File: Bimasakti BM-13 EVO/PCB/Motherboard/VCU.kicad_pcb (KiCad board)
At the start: 2 copper layers, 190.7 x 210 mm, 27 parts, among them J1 6437288-3, J10 power, J11 6437288-3, J2 12V, J3 3V3_1, J4 5V_5, J5 5V_1, J6 5V_2, J7 5V_3, J8 SIGNAL 1, J9 SIGNAL 2

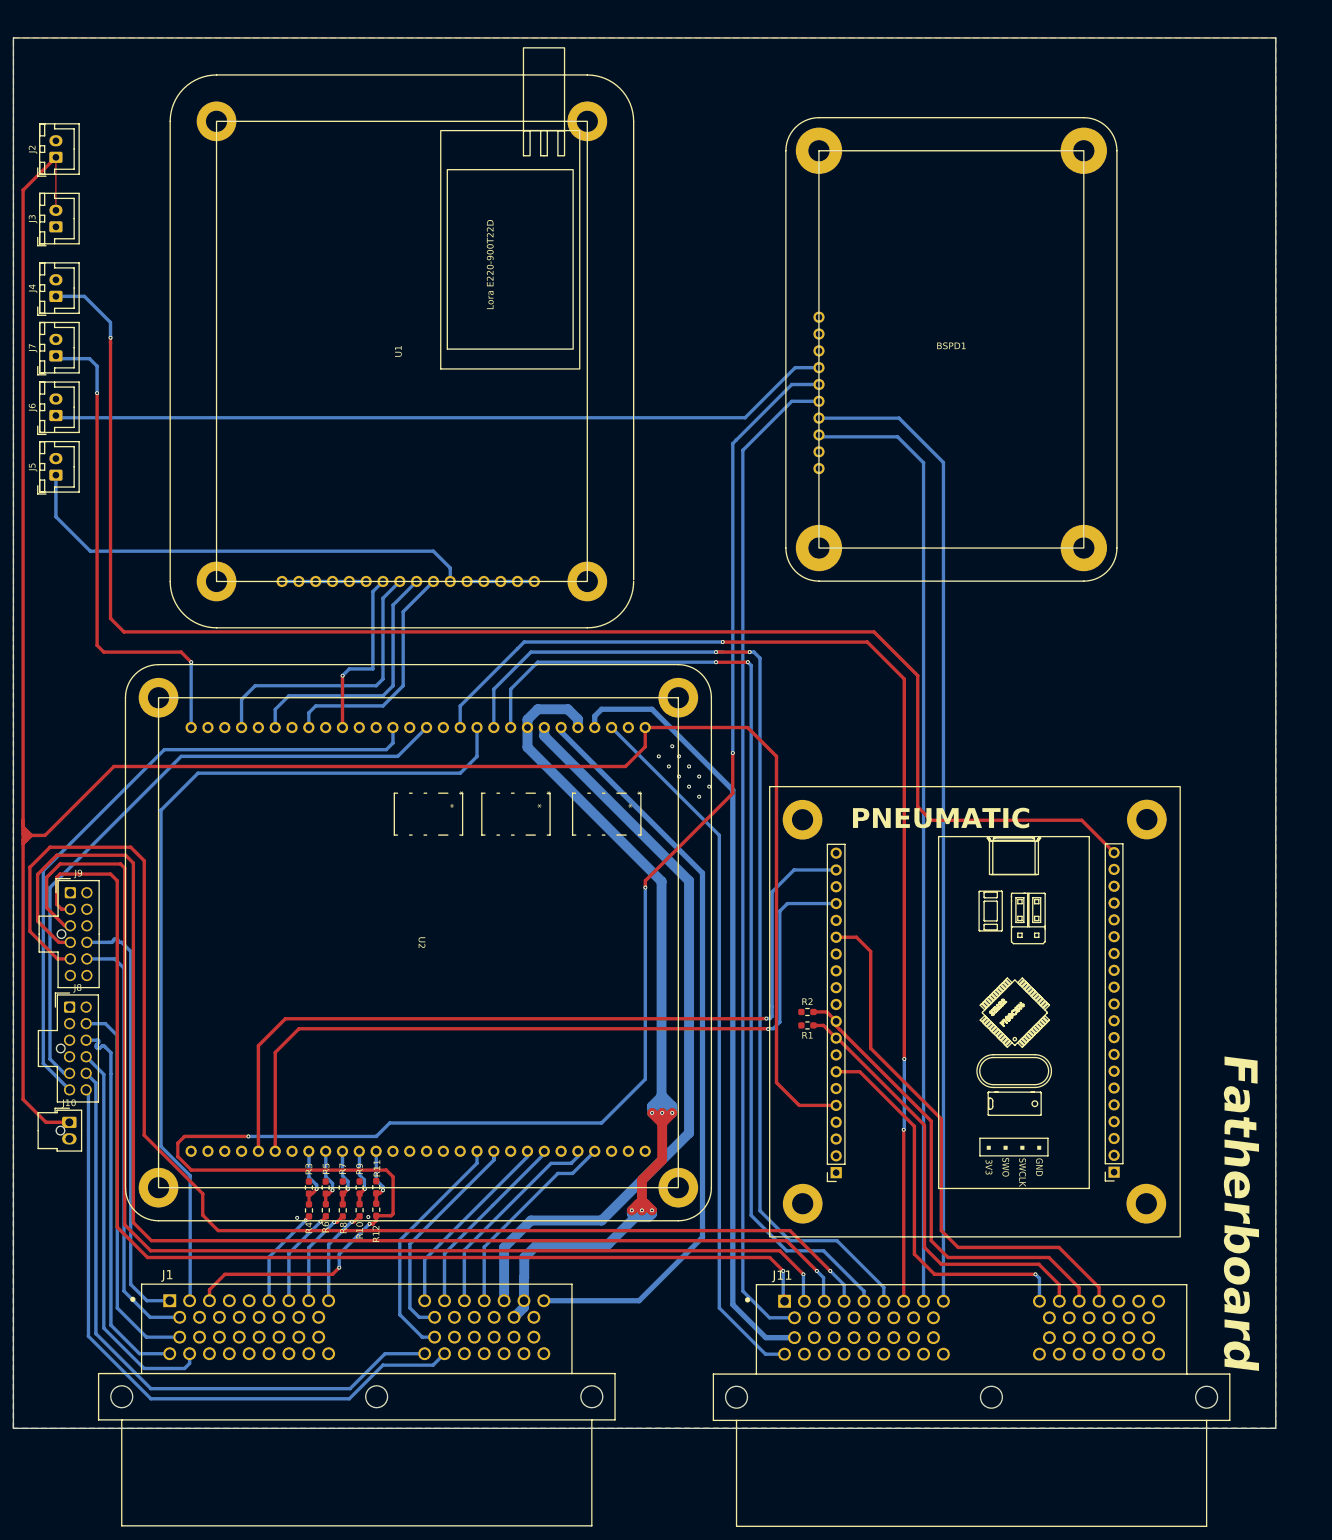
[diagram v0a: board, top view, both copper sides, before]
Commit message: Asu
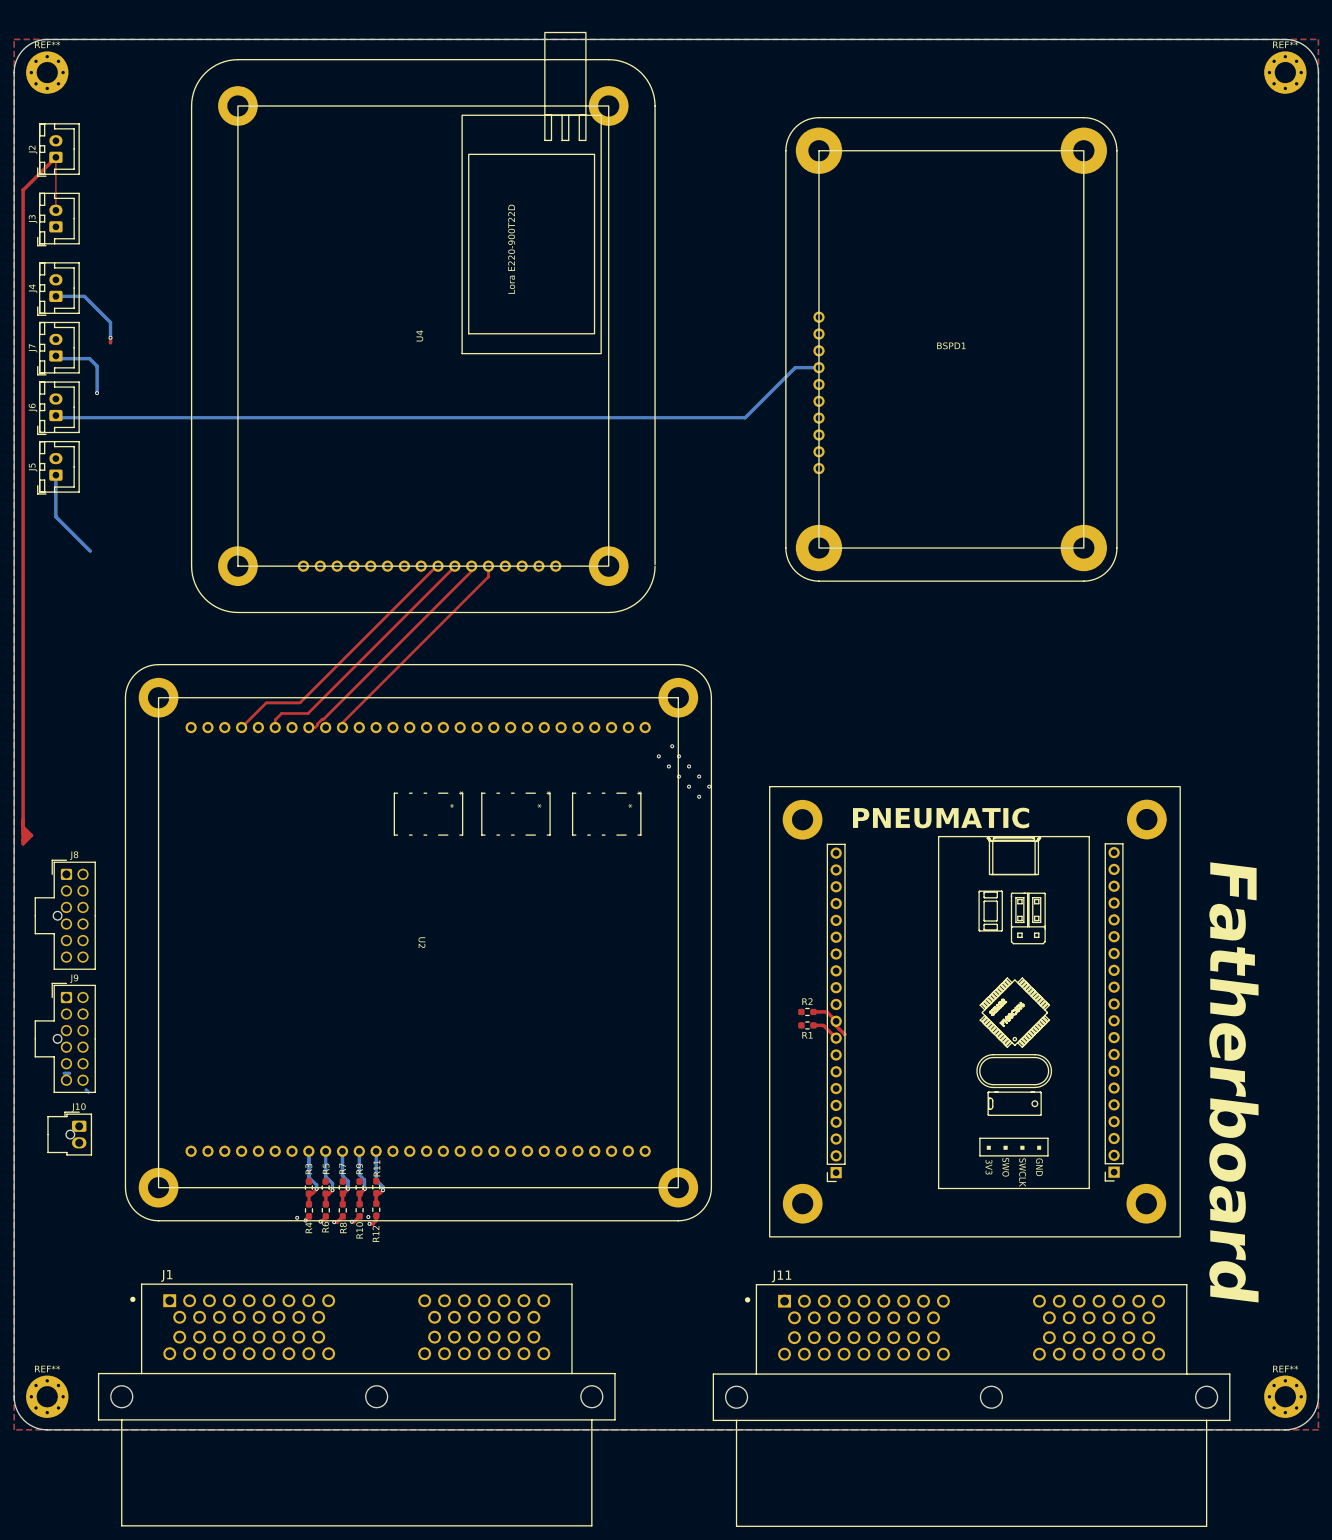
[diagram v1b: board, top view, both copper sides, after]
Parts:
- removed U1: ~, 0_FootprintTelemetry:0_FootprintTelemetry
- added REF**: MountingHole_3.2mm_M3_Pad_Via, MountingHole:MountingHole_3.2mm_M3_Pad_Via, F.Cu at (340.0, 105.0)
- added REF**: MountingHole_3.2mm_M3_Pad_Via, MountingHole:MountingHole_3.2mm_M3_Pad_Via, F.Cu at (153.0, 105.0)
- added REF**: MountingHole_3.2mm_M3_Pad_Via, MountingHole:MountingHole_3.2mm_M3_Pad_Via, F.Cu at (153.0, 305.0)
- added REF**: MountingHole_3.2mm_M3_Pad_Via, MountingHole:MountingHole_3.2mm_M3_Pad_Via, F.Cu at (340.0, 305.0)
- added U4: ~, 0_FootprintTelemetry:0_FootprintTelemetry, F.Cu at (209.8, 144.8)
- moved J8 20.1 mm to (155.9, 226.1)
- moved J9 15.8 mm to (155.9, 244.7)
- moved J10 1.60 mm to (157.8, 264.1)
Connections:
- BSPD1 pad 3: NC -> SDC_B
- BSPD1 pad 4: COM -> SDC_OUT
- J1 pad 11: BAT_FAN -> unconnected-(J1-Pad11)
- J1 pad 17: unconnected-(J1-Pad17) -> IND_SWITCH
- J1 pad 21: BMS_CAN -> unconnected-(J1-Pad21)
- J1 pad 28: COM_BSPD -> unconnected-(J1-Pad28)
- J1 pad 29: NC_BSPD -> unconnected-(J1-Pad29)
- J11 pad 8: NC -> unconnected-(J11-Pad8)
- J11 pad 9: COM -> unconnected-(J11-Pad9)
- U2 pad 10: SDC_OUT -> SDC_B
- U2 pad 27: unconnected-(U2-SWITCH-Pad27) -> IND_SWITCH
- U2 pad 29: unconnected-(U2-+5V-Pad29) -> 5V_V
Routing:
- net BRK_P: track 269.9 -> 1.87 mm, vias 5 -> 1
- net 12V: track 343.8 -> 114.2 mm
- net 5V_P: track 232.4 -> 12.9 mm
- net WS_FR: track 197.8 -> 0.00 mm, vias 1 -> 0
- net WS_FL: track 195.1 -> 0.14 mm, vias 1 -> 0
- net WS_RR: track 185.8 -> 0.21 mm, vias 1 -> 0
- net WS_RL: track 177.3 -> 1.10 mm, vias 1 -> 0
- net FAN_BATT: track 170.7 -> 0.00 mm, vias 3 -> 0
- net SDC_OUT: track 159.8 -> 0.82 mm, vias 2 -> 0
- net TPS: track 151.0 -> 0.00 mm
- net SDC_IN: track 150.4 -> 0.00 mm, vias 2 -> 0
- net COM: track 148.3 -> 0.00 mm
- net NC: track 144.2 -> 0.00 mm
- net SAFETY: track 143.4 -> 0.00 mm, vias 6 -> 0
- net BRAKE_LIGHT: track 131.4 -> 0.12 mm
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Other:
- board size 190.7 x 210 mm -> 197 x 210 mm

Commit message: vcu lebih rapi
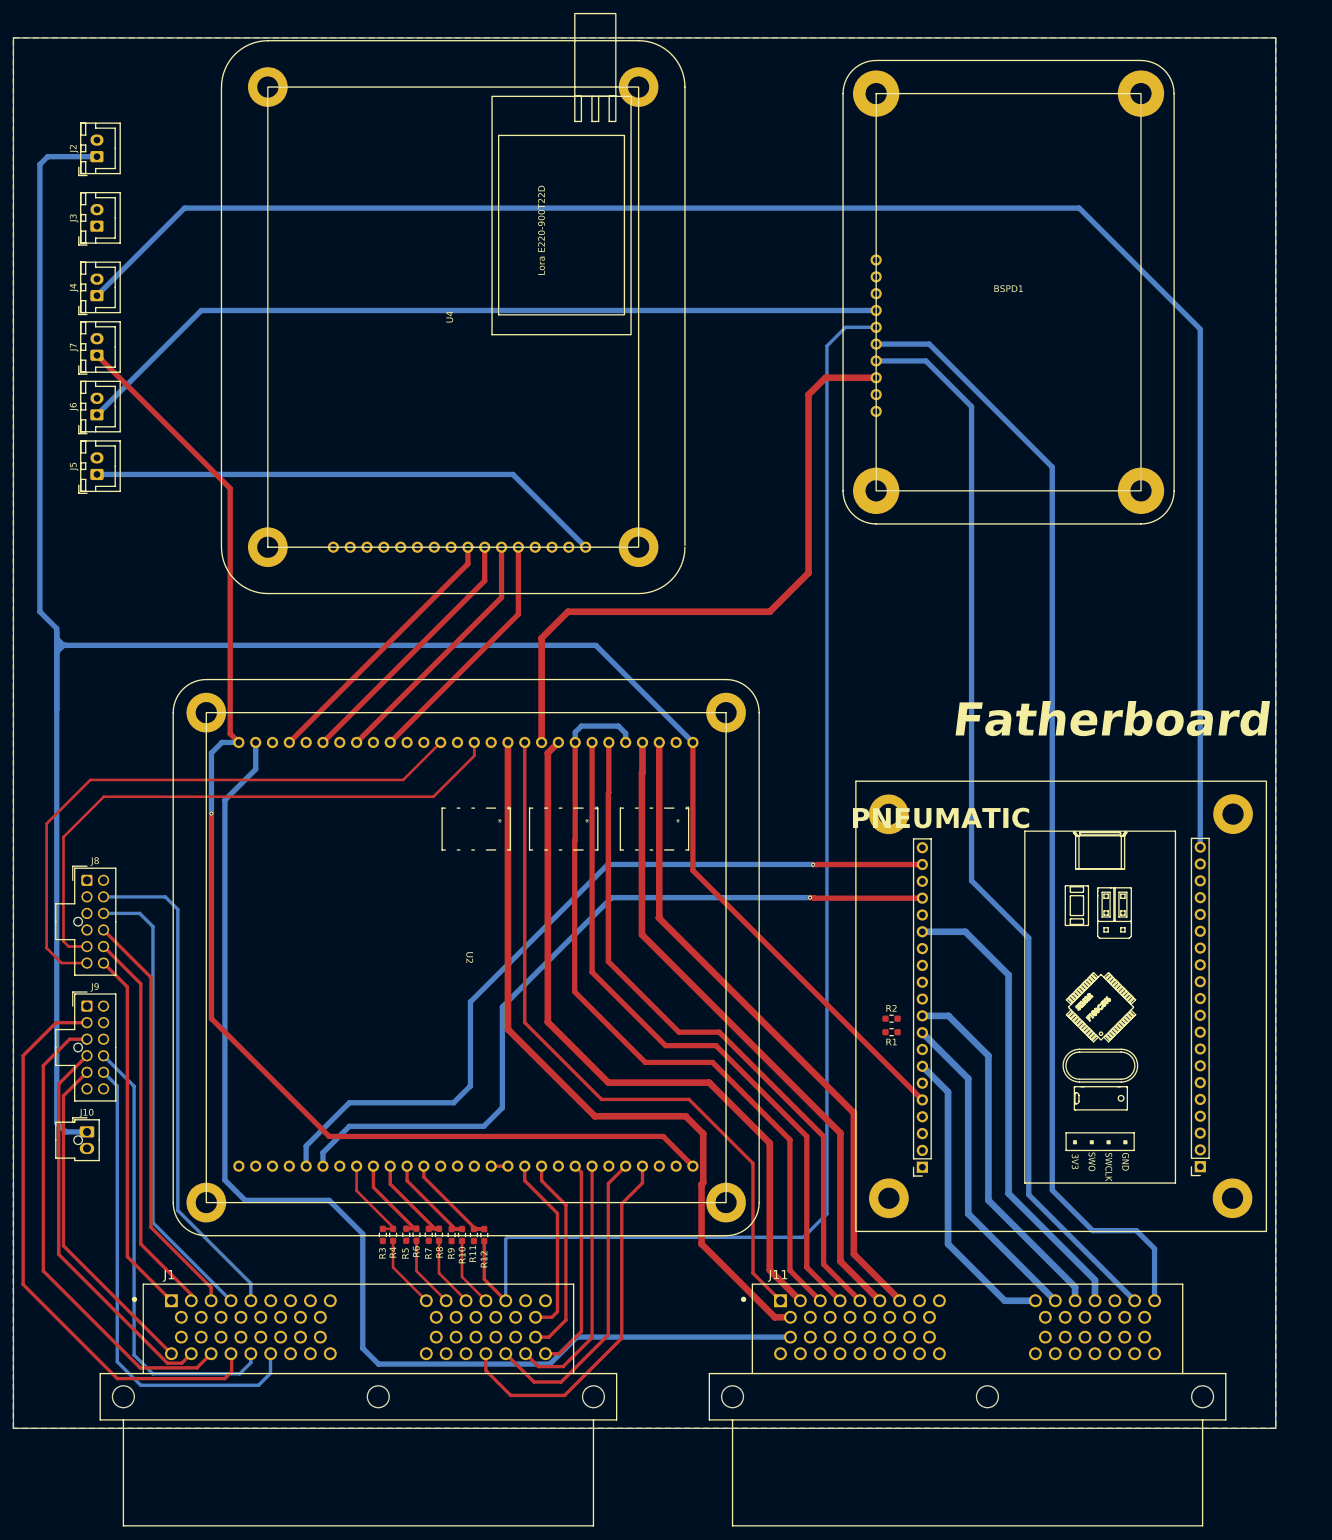
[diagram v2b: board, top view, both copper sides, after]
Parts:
- removed REF** (x4): MountingHole_3.2mm_M3_Pad_Via, MountingHole:MountingHole_3.2mm_M3_Pad_Via
- moved R12 16.8 mm to (219.0, 280.6)
- moved R11 16.4 mm to (217.4, 280.6), turned to -90 degrees
- moved R10 15.9 mm to (215.6, 280.6)
- moved R9 15.6 mm to (214.1, 280.6), turned to -90 degrees
- moved R8 15.0 mm to (212.2, 280.5)
- moved R7 14.8 mm to (210.6, 280.5), turned to -90 degrees
- moved R6 14.2 mm to (208.8, 280.5)
- moved R5 14.1 mm to (207.2, 280.5), turned to -90 degrees
- moved R3 13.3 mm to (203.7, 280.6), turned to -90 degrees
- moved R4 13.2 mm to (205.2, 280.6)
- moved U3 13.0 mm to (306.1, 243.4)
- moved R1 12.7 mm to (280.5, 249.9)
- moved R2 12.7 mm to (280.5, 247.9)
- moved BSPD1 12.2 mm to (298.2, 138.2)
- moved U2 7.56 mm to (216.3, 238.7)
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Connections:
- J1 pad 1: ESC2_LO -> APPS_IN1
- J1 pad 10: ESC2_HI -> unconnected-(J1-Pad10)
- J1 pad 17: IND_SWITCH -> unconnected-(J1-Pad17)
- J1 pad 18: ESC1_LO -> unconnected-(J1-Pad18)
- J1 pad 2: BRAKE_LIGHT -> APPS_IN2
- J1 pad 26: ESC1_HI -> WS_FR
- J1 pad 27: STEER_IN -> WS_FL
- J1 pad 28: unconnected-(J1-Pad28) -> WS_RR
- J1 pad 29: unconnected-(J1-Pad29) -> WS_RL
- J1 pad 3: BRK_P -> STEER_IN
- J1 pad 30: unconnected-(J1-Pad30) -> ESC2_LO
- J1 pad 31: unconnected-(J1-Pad31) -> ESC2_HI
- J1 pad 35: BMS_LO -> SUSP1
- J1 pad 36: BMS_HI -> SUSP2
- J1 pad 37: ECU_LO -> SUSP3
- J1 pad 38: ECU_HI -> SUSP4
- J1 pad 39: AIR -> BRK_P
- J1 pad 4: unconnected-(J1-Pad4) -> ESC1_HI
- J1 pad 40: SAFETY -> unconnected-(J1-Pad40)
- J1 pad 41: SWITCH_HY -> unconnected-(J1-Pad41)
- J1 pad 42: DISP_HI -> unconnected-(J1-Pad42)
- J1 pad 46: SAFETY -> unconnected-(J1-Pad46)
- J1 pad 47: unconnected-(J1-Pad47) -> DISP_LO
- J1 pad 48: DISP_LO -> unconnected-(J1-Pad48)
- J1 pad 5: GND -> ESC1_LO
- J1 pad 53: unconnected-(J1-Pad53) -> DISP_HI
- J1 pad 54: APPS_IN2 -> unconnected-(J1-Pad54)
- J1 pad 55: APPS_IN1 -> unconnected-(J1-Pad55)
- J1 pad 57: unconnected-(J1-Pad57) -> ECU_HI
- J1 pad 58: GPOS -> ECU_LO
- J1 pad 59: unconnected-(J1-Pad59) -> BMS_HI
- J1 pad 6: SUSP1 -> unconnected-(J1-Pad6)
- J1 pad 60: unconnected-(J1-Pad60) -> BMS_LO
- J1 pad 7: SUSP2 -> unconnected-(J1-Pad7)
- J1 pad 8: SUSP3 -> unconnected-(J1-Pad8)
- J1 pad 9: SUSP4 -> unconnected-(J1-Pad9)
- J11 pad 1: WS_RL -> BRAKE_LIGHT
- J11 pad 10: TPS -> FAN_BATT
- J11 pad 18: PDM -> IND_SWITCH
- J11 pad 2: WS_RR -> SDC_IN
- J11 pad 26: ENG_RLY -> unconnected-(J11-Pad26)
- J11 pad 3: WS_FL -> SAFETY
- J11 pad 39: unconnected-(J11-Pad39) -> GPOS
- J11 pad 4: WS_FR -> AIR
- J11 pad 40: unconnected-(J11-Pad40) -> SDC_OUT
- J11 pad 41: unconnected-(J11-Pad41) -> TPS
- J11 pad 5: SDC_IN -> SWITCH_HY
- J11 pad 6: SDC_OUT -> PDM
- J11 pad 7: FAN_BATT -> ENG_RLY
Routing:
- net 5V_P: track 12.9 -> 257.9 mm, vias 1 -> 0
- net 12V: track 114.2 -> 347.6 mm
- net BRK_P: track 1.87 -> 209.4 mm, vias 1 -> 0
- net 5V_V: track 10.9 -> 194.2 mm
- net IND_SWITCH: track 0.00 -> 176.8 mm
- net TPS: track 0.00 -> 170.5 mm
- net SDC_OUT: track 0.82 -> 162.5 mm
- net TX_PNEU: track 0.00 -> 121.2 mm, vias 0 -> 1
- net RX_PNEU: track 0.00 -> 117.5 mm, vias 0 -> 1
- net SAFETY: track 0.00 -> 117.0 mm
- net FAN_BATT: track 0.00 -> 114.1 mm
- net SDC_IN: track 0.00 -> 110.5 mm
- net BRAKE_LIGHT: track 0.12 -> 108.1 mm
- net AIR: track 0.00 -> 104.3 mm
- net SWITCH_HY: track 0.00 -> 103.7 mm
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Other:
- board size 197 x 210 mm -> 190.7 x 210 mm
